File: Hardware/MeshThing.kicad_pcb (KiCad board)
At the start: 4 copper layers, 19.1 x 24.7 mm, 22 parts, among them IC1 ATMEGA2564/1284/644RFR2, P1 CONN34

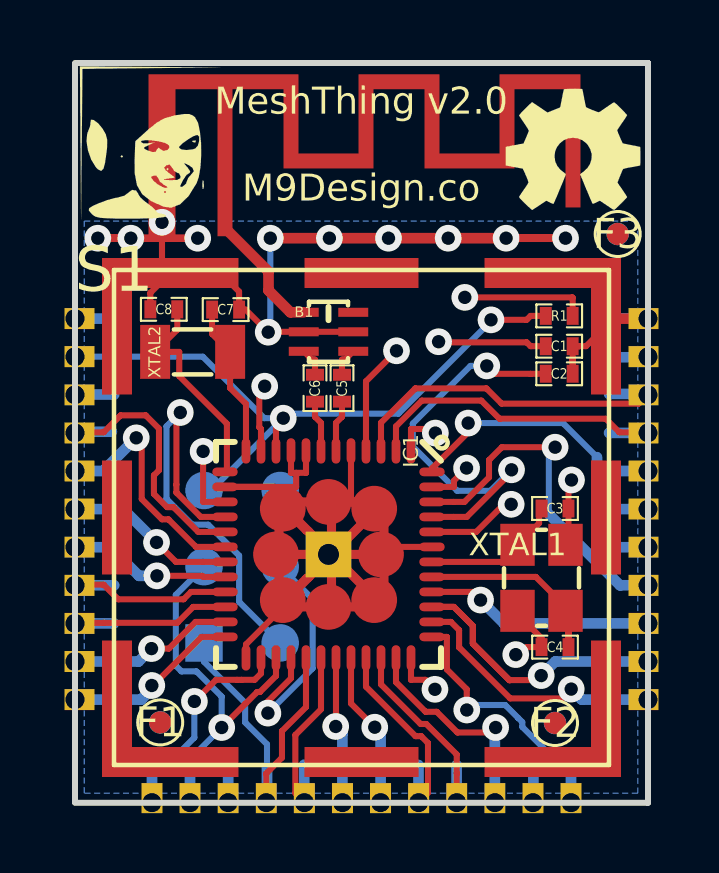
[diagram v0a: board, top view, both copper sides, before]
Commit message: Very nearly there.
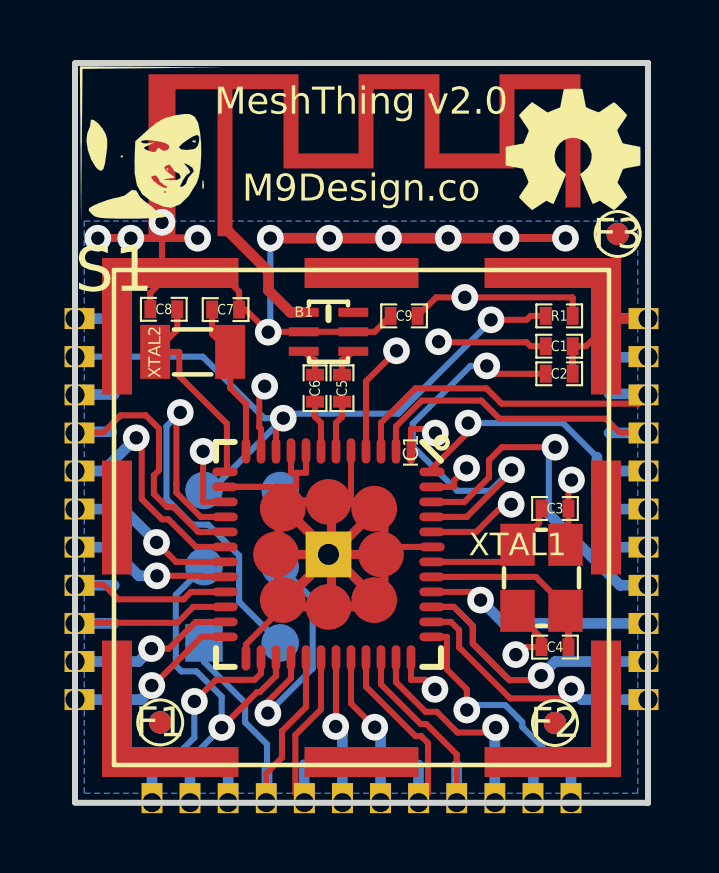
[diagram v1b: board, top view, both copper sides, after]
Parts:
- added C9: 100n, SMD_Packages:SM0402_c, F.Cu at (151.4, 96.1)
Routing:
- net +3.3V: track 59.2 -> 61.1 mm
- net GND: track 94.8 -> 96.3 mm
